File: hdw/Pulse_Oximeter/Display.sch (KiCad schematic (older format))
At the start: 21 parts, among them U1601 74LVC1G17, U1602 NHD-0420H1Z

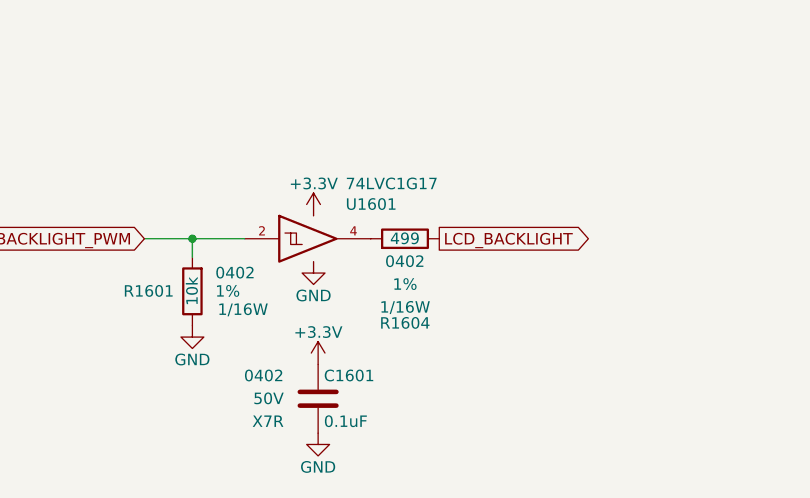
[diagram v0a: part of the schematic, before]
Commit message: added deployable BOM
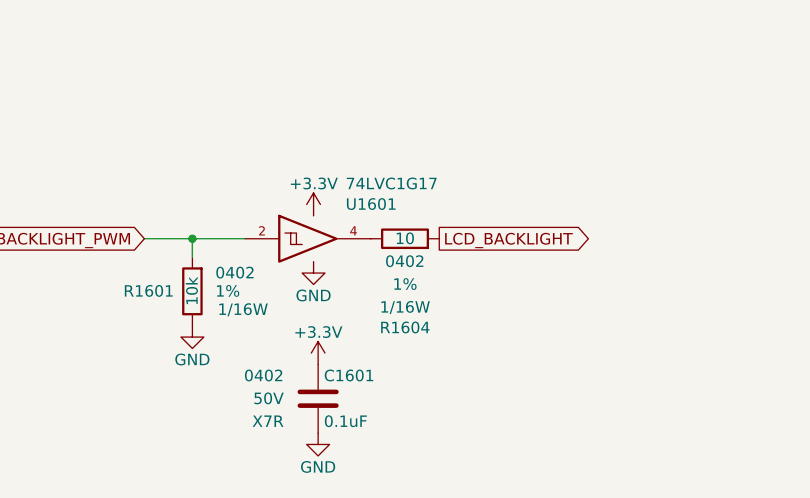
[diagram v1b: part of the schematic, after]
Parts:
- R1604: value 499 -> 10; Digi-Key PN RMCF0402FT499RCT-ND -> 541-3964-1-ND
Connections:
- net LCD_BACKLIGHT: now also R1604.1; no longer R1604.2
- net at U1601.4: now also R1604.2; no longer R1604.1
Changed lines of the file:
@@
 	1    0    0    -1
-$EndComp
-$Comp
-L Custom_Library:R_Custom R?
-U 1 1 5EB2CCF7
-P 3730 6230
-AR Path="/5CB6F1ED/5EB2CCF7" Ref="R?"  Part="1"
-AR Path="/5CB7718D/5EB2CCF7" Ref="R?"  Part="1"
-AR Path="/5E0DC082/5EB2CCF7" Ref="R?"  Part="1"
-AR Path="/5E0F263A/5EB2CCF7" Ref="R?"  Part="1"
-AR Path="/5EAE2D8A/5EB2CCF7" Ref="R?"  Part="1"
-AR Path="/5EAE2E5F/5EB2CCF7" Ref="R?"  Part="1"
-AR Path="/5EAE4A89/5EB2CCF7" Ref="R1604"  Part="1"
-F 0 "R1604" V 4100 6230 50  0000 C CNN
-F 1 "499" V 3730 6230 50  0000 C CNN
-F 2 "Resistors_SMD:R_0402" H 3730 6230 50  0001 C CNN
-F 3 "" H 3730 6230 50  0001 C CNN
-F 4 "0402" V 3830 6230 50  0000 C CNN "display_footprint"
-F 5 "1%" V 3930 6230 50  0000 C CNN "Tolerance"
-F 6 "1/16W" V 4030 6230 50  0000 C CNN "Wattage"
-F 7 "RMCF0402FT499RCT-ND" H 3730 6230 50  0001 C CNN "Digi-Key PN"
-	1    3730 6230
-	0    -1   1    0
 $EndComp
 Text GLabel 3880 6230 2    50   Output ~ 0
@@
 Wire Wire Line
 	4860 4520 5190 4520
+$Comp
+L Custom_Library:R_Custom R?
+U 1 1 5F1BFFAE
+P 3730 6230
+AR Path="/5EAE2D66/5F1BFFAE" Ref="R?"  Part="1"
+AR Path="/5EAE4A89/5F1BFFAE" Ref="R1604"  Part="1"
+F 0 "R1604" V 4120 6230 50  0000 C CNN
+F 1 "10" V 3730 6230 50  0000 C CNN
+F 2 "Resistors_SMD:R_0402" H 3730 6230 50  0001 C CNN
+F 3 "" H 3730 6230 50  0001 C CNN
+F 4 "541-3964-1-ND" H 4030 6630 60  0001 C CNN "Digi-Key PN"
+F 5 "0402" V 3830 6230 50  0000 C CNN "display_footprint"
+F 6 "1%" V 3930 6230 50  0000 C CNN "Tolerance"
+F 7 "1/16W" V 4030 6230 50  0000 C CNN "Wattage"
+	1    3730 6230
+	0    1    1    0
+$EndComp
 $EndSCHEMATC
